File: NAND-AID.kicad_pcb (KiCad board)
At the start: 2 copper layers, 33.7 x 21.4 mm, 24 parts

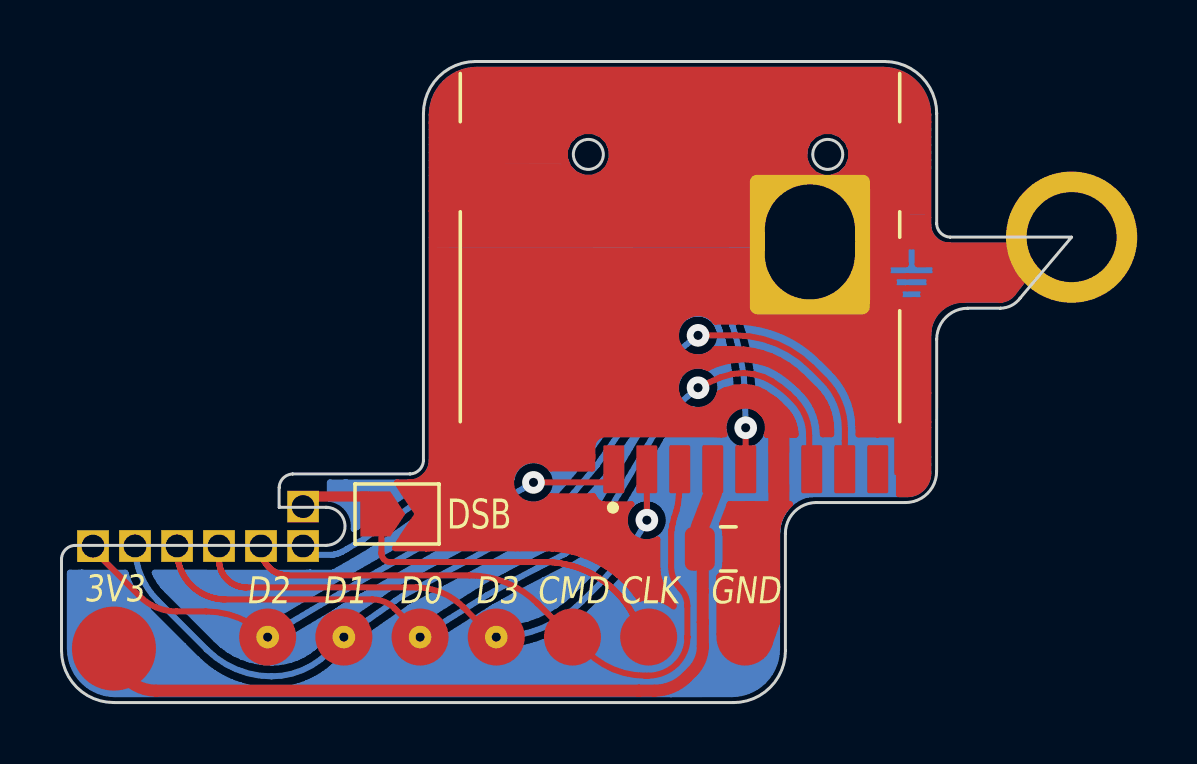
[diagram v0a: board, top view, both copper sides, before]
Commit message: Small fixes
Signed-off-by: Thomas Rohloff <v10lator@myway.de>
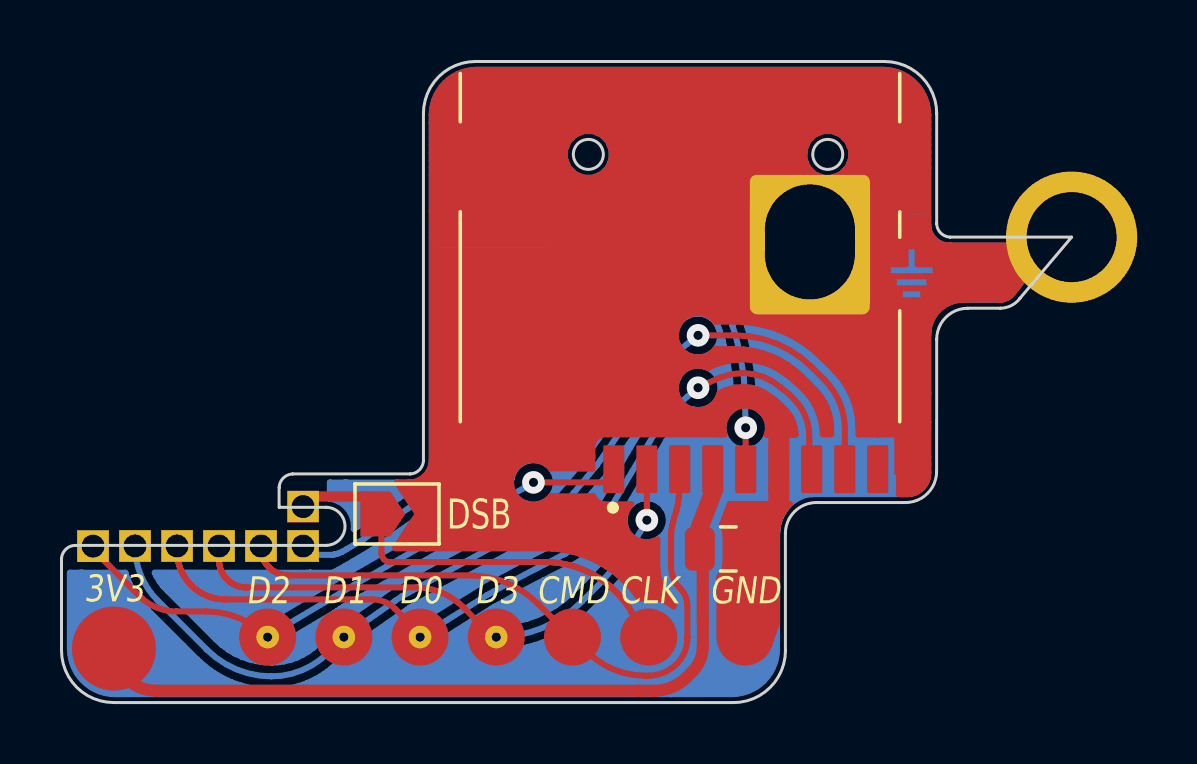
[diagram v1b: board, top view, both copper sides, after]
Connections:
- ? pad : (no net) -> 3V3
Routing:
- net GND: track 3438.7 -> 3447.8 mm
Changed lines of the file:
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@@
         (effects (font (size 1 1) (thickness 0.15)))
     )
-    (pad "" smd circle (at -1.3 0) (size 2.8 2.8) (layers "F.Cu" "F.Paste" "F.Mask"))
+    (pad "" smd circle (at -1.3 0) (size 2.8 2.8) (layers "F.Cu" "F.Paste" "F.Mask")
+      (net 1 "3V3"))
   )
   (footprint "" (layer "F.Cu")
@@
   (segment (start 157.106075 92.544313) (end 158.430969 92.544313) (width 0.2) (layer "F.Cu") (net 2))
   (segment (start 146.360586 105.206521) (end 145.897971 105.213358) (width 0.2) (layer "F.Cu") (net 2))
+  (segment (start 145.836806 96.738042) (end 152.565118 96.753368) (width 0.2) (layer "F.Cu") (net 2))
   (segment (start 158.430999 92.584481) (end 158.430999 92.324349) (width 0.2) (layer "F.Cu") (net 2))
   (segment (start 159.138943 97.587672) (end 158.934973 97.791892) (width 0.2) (layer "F.Cu") (net 2))
@@
   (segment (start 153.704 105.407315) (end 152.469736 105.459617) (width 0.2) (layer "F.Cu") (net 2))
   (segment (start 146.890656 106.521389) (end 146.928942 106.625306) (width 0.2) (layer "F.Cu") (net 2))
+  (segment (start 143.90136 93.972647) (end 146.283613 93.987352) (width 0.2) (layer "F.Cu") (net 2))
   (segment (start 153.172618 99.395978) (end 153.555071 99.533133) (width 0.2) (layer "F.Cu") (net 2))
   (segment (start 146.64512 94.329) (end 146.94103 94.45168) (width 0.254) (layer "F.Cu") (net 2))
